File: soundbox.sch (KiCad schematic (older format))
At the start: 180 parts, among them J10 COLOR INPUT, J11 MONO INPUT, J12 NEXT PWR INPUT 1, J13 NEXT PWR INPUT 2, J14 -12VDC OUT, J15 5VDC STANDBY, J16 MON IN 1, J17 MON IN 2, J18 PA1, J19 BOOT0, J2 OUT (SJ1-3535NG), J20 PC0, J21 PC1, J22 PB0, J23 PB1, J24 R SPK, J25 R SPEAKER (SJ-2509N), J26 L SPEAKER, J27 L SPK, J28 I2C Ext, J29 OLED, J3 MIC (SJ1-3535NG), J31 NeXT Keyboard, J32 NeXT Keyboard (MD-50SM / KMDG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, J4 USB Host (SS-52100-001), J5 Mic IN, J6 Audio OUT, J7 STLINK, J8 UART2, J9 PA0, Q1 2SC2712, SW1 NeXT POWER SW (1-1825027-1 / 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, SW3 NeXT POWER SW, SW4 MCU RESET, U11 TLV70033DDCR, U17 USBLC6-2SC6, U18 STMPS2141STR, U19 SN74LVC2G34DBV, U20 PCM5122PW, U21 TLV70033DDCR (or XC6204B332MR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, U22 TLV70033DDCR (or XC6204B332MR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, U23 PLT133/T, U24 STM32F401RCT6, U25 SN74LVC1G07DBV, U26 SN74HCT125DR, U27 TLV320ADC3100, U28 BD33FC0FP, U29 TPA2005D1DGN, U30 BD33FC0FP, U31 TPA2005D1DGN, U32 PCA9515D, U8 5V(DC/DC), X3 ECS-2520MVLC-225.792-BN-TR, Y2 25MHz (FA-238 25.0000MB-K0)

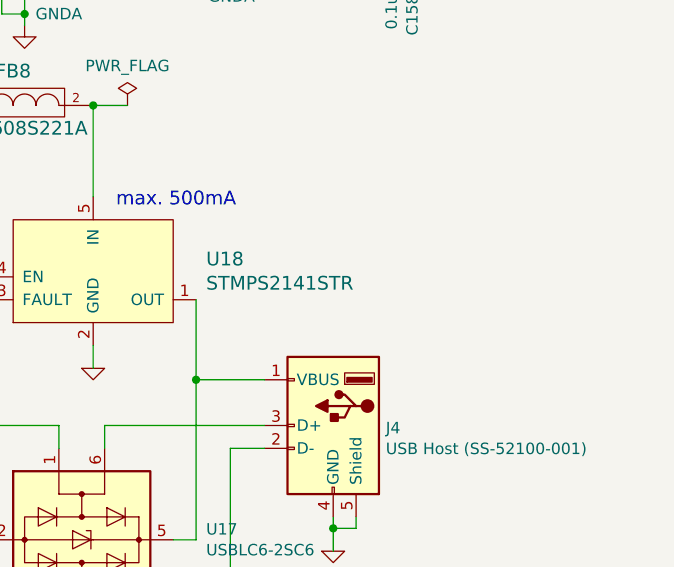
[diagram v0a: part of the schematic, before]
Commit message: update position
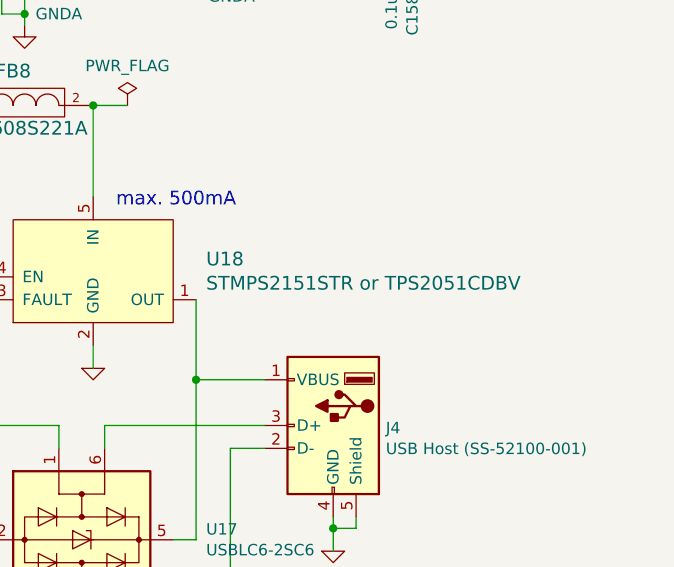
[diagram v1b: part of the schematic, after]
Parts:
- U18: value STMPS2141STR -> STMPS2151STR‎ or TPS2051CDBV
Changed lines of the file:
@@
 P 13850 6550
 F 0 "U18" H 14344 6828 60  0000 L CNN
-F 1 "STMPS2141STR" H 14344 6722 60  0000 L CNN
+F 1 "STMPS2151STR‎ or TPS2051CDBV" H 14344 6722 60  0000 L CNN
 F 2 "Package_TO_SOT_SMD:SOT-23-5_HandSoldering" H 13850 6550 60  0001 C CNN
 F 3 "" H 13850 6550 60  0001 C CNN
